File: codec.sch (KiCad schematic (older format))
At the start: 15 parts, among them U4 TLV320AIC3101

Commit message: Use a better codec
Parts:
- removed TP1: MIC1LP/LINE1LP, symbol Connector:TestPoint_Probe
- removed TP2: HPLCOM, symbol Connector:TestPoint_Probe
- removed TP3: HPLOUT, symbol Connector:TestPoint_Probe
- removed TP4: LEFT_LOM, symbol Connector:TestPoint_Probe
- removed TP5: LEFT_LOP, symbol Connector:TestPoint_Probe
- removed U4: TLV320AIC3101, Package_DFN_QFN:QFN-32-1EP_5x5mm_P0.5mm_EP3.65x3.65mm, symbol Audio:TLV320AIC3101
- added C13: 0.1u, symbol Device:C
- added C14: 1u, symbol Device:C
- added C15: 10u, symbol Device:C
- added U2: WM8731SEDS, Package_SO:SSOP-28_5.3x10.2mm_P0.65mm, symbol Audio:WM8731SEDS
- C10, C12: value 1u -> 10u
- C11: value 0.1u -> 10u
- C6: value 1u -> 0.1u
- C8: value 10u -> 1u
- C9: value 0.1u -> 1u
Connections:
- net labels added: ADC, AVDD, DAC, DBVDD, DCVDD, HPVDD, SCLK, SDIN, ~CSB
- net labels removed: 1.8V, DIN, DOUT, SCL, SDA, ~RESET
- no-connect marks 10 -> 9

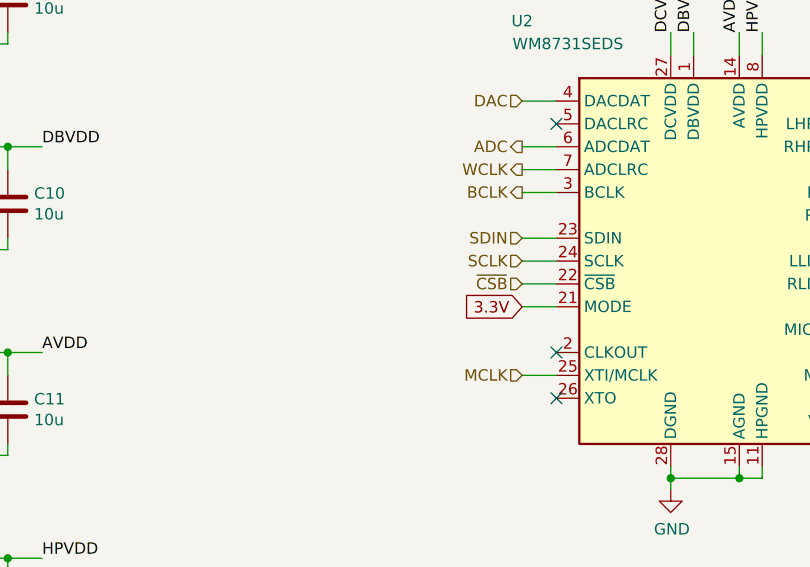
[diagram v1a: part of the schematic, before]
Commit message: Various fixes
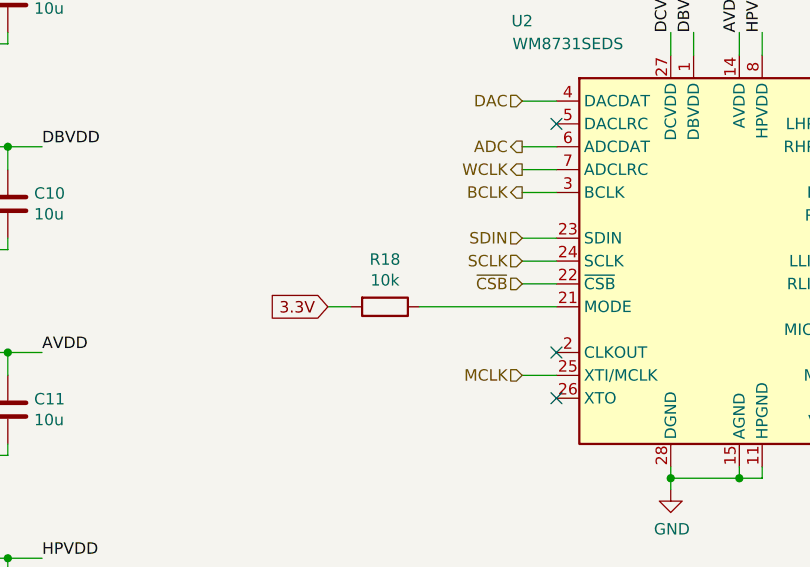
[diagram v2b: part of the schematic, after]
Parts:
- added R18: 10k, symbol Device:R
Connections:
- net 3.3V: now also R18.2; no longer U2.21 (MODE)
- new net: R18.1, U2.21 (MODE)
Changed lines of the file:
@@
 Wire Wire Line
 	5250 3950 5400 3950
-Text GLabel 5250 4250 0    50   Input ~ 0
-3.3V
-Wire Wire Line
-	5250 4250 5400 4250
+Text GLabel 4400 4250 0    50   Input ~ 0
+3.3V
 Text GLabel 1950 2650 0    50   Input ~ 0
 3.3V
@@
 Wire Wire Line
 	6300 3050 6300 3150
+$Comp
+L Device:R R18
+U 1 1 6039A986
+P 4650 4250
+F 0 "R18" V 4443 4250 50  0000 C CNN
+F 1 "10k" V 4534 4250 50  0000 C CNN
+F 2 "" V 4580 4250 50  0001 C CNN
+F 3 "~" H 4650 4250 50  0001 C CNN
+	1    4650 4250
+	0    1    1    0
+$EndComp
+Wire Wire Line
+	4500 4250 4400 4250
+Wire Wire Line
+	4800 4250 5400 4250
 $EndSCHEMATC
